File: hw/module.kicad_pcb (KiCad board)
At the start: 2 copper layers, 30 x 30 mm, 1 part

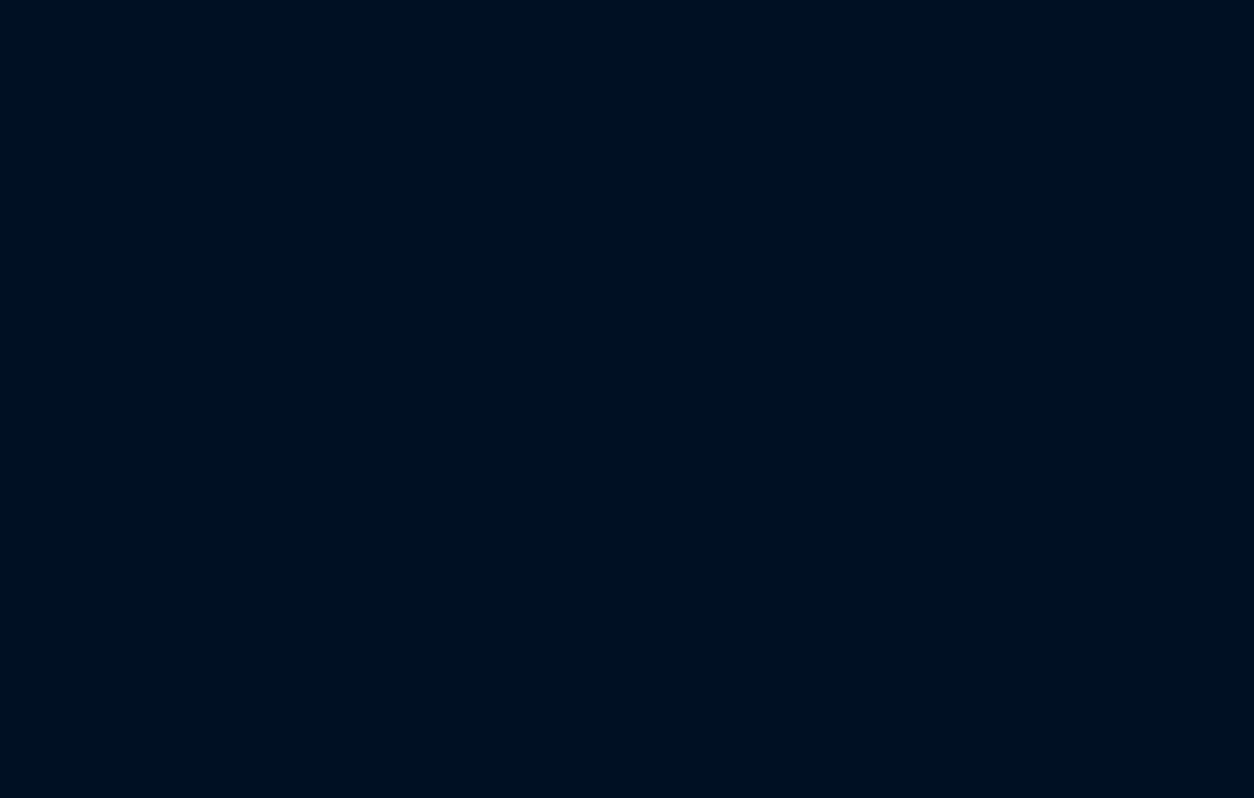
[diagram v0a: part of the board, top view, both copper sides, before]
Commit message: Footprint assignment
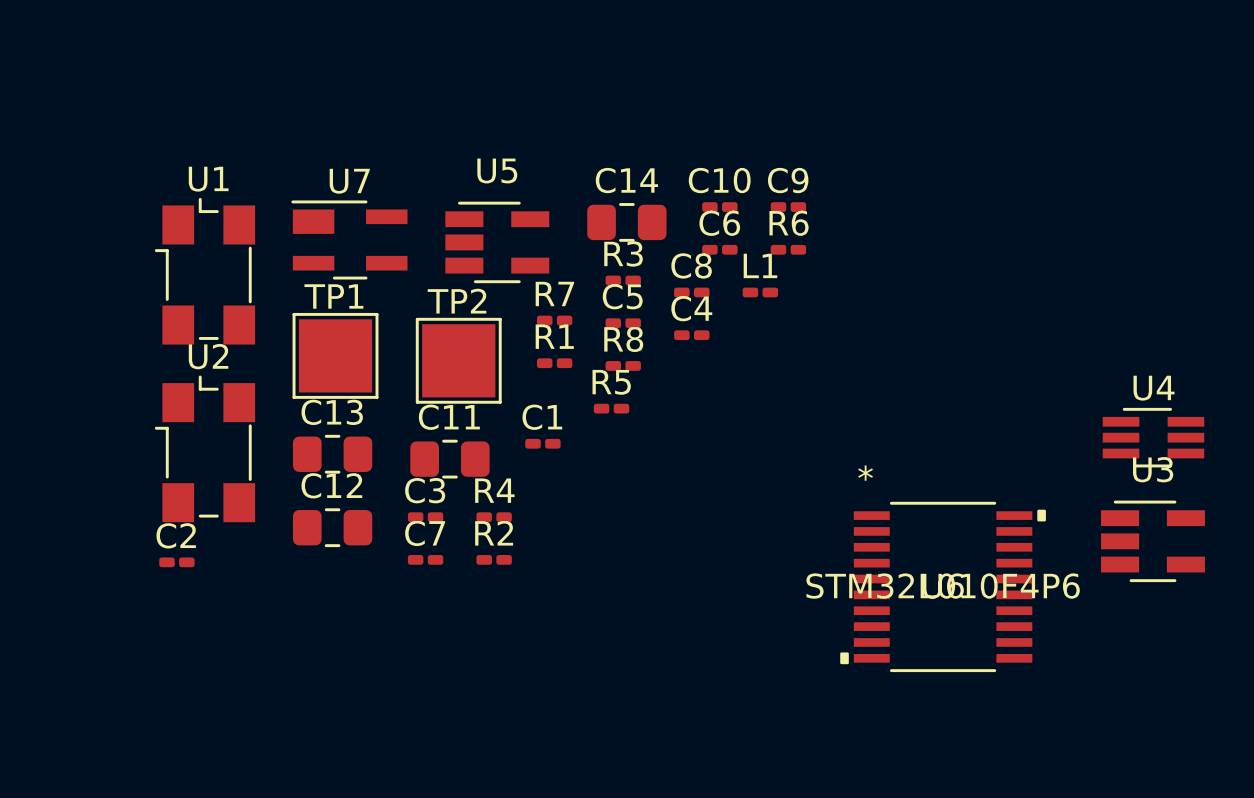
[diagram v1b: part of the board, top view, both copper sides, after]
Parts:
- added C1: 10n, Capacitor_SMD:C_0201_0603Metric_Pad0.64x0.40mm_HandSolder, F.Cu at (99.5, 62.5)
- added C10: 10n, Capacitor_SMD:C_0201_0603Metric_Pad0.64x0.40mm_HandSolder, F.Cu at (106.8, 52.8)
- added C11: 100n, Capacitor_SMD:C_0805_2012Metric_Pad1.18x1.45mm_HandSolder, F.Cu at (95.7, 63.1)
- added C12: 100n, Capacitor_SMD:C_0805_2012Metric_Pad1.18x1.45mm_HandSolder, F.Cu at (90.9, 65.9)
- added C13: 100n, Capacitor_SMD:C_0805_2012Metric_Pad1.18x1.45mm_HandSolder, F.Cu at (90.9, 62.9)
- added C14: 100n, Capacitor_SMD:C_0805_2012Metric_Pad1.18x1.45mm_HandSolder, F.Cu at (102.9, 53.4)
- added C2: 10n, Capacitor_SMD:C_0201_0603Metric_Pad0.64x0.40mm_HandSolder, F.Cu at (84.5, 67.4)
- added C3: 100n, Capacitor_SMD:C_0201_0603Metric_Pad0.64x0.40mm_HandSolder, F.Cu at (94.7, 65.5)
- added C4: 100n, Capacitor_SMD:C_0201_0603Metric_Pad0.64x0.40mm_HandSolder, F.Cu at (105.6, 58.0)
- added C5: 200p, Capacitor_SMD:C_0201_0603Metric_Pad0.64x0.40mm_HandSolder, F.Cu at (102.8, 57.6)
- added C6: 200p, Capacitor_SMD:C_0201_0603Metric_Pad0.64x0.40mm_HandSolder, F.Cu at (106.8, 54.5)
- added C7: 10n, Capacitor_SMD:C_0201_0603Metric_Pad0.64x0.40mm_HandSolder, F.Cu at (94.7, 67.3)
- added C8: 100n, Capacitor_SMD:C_0201_0603Metric_Pad0.64x0.40mm_HandSolder, F.Cu at (105.6, 56.3)
- added C9: 100n, Capacitor_SMD:C_0201_0603Metric_Pad0.64x0.40mm_HandSolder, F.Cu at (109.6, 52.8)
- added L1: L, Inductor_SMD:L_0201_0603Metric_Pad0.64x0.40mm_HandSolder, F.Cu at (108.4, 56.3)
- added R1: 10k, Resistor_SMD:R_0201_0603Metric_Pad0.64x0.40mm_HandSolder, F.Cu at (100.0, 59.2)
- added R2: 10k, Resistor_SMD:R_0201_0603Metric_Pad0.64x0.40mm_HandSolder, F.Cu at (97.5, 67.3)
- added R3: 800k, Resistor_SMD:R_0201_0603Metric_Pad0.64x0.40mm_HandSolder, F.Cu at (102.8, 55.8)
- added R4: 800k, Resistor_SMD:R_0201_0603Metric_Pad0.64x0.40mm_HandSolder, F.Cu at (97.5, 65.5)
- added R5: R, Resistor_SMD:R_0201_0603Metric_Pad0.64x0.40mm_HandSolder, F.Cu at (102.3, 61.1)
- added R6: 500k, Resistor_SMD:R_0201_0603Metric_Pad0.64x0.40mm_HandSolder, F.Cu at (109.6, 54.5)
- added R7: 500k, Resistor_SMD:R_0201_0603Metric_Pad0.64x0.40mm_HandSolder, F.Cu at (100.0, 57.5)
- added R8: 10k, Resistor_SMD:R_0201_0603Metric_Pad0.64x0.40mm_HandSolder, F.Cu at (102.8, 59.3)
- added TP1: SWDIO, TestPoint:TestPoint_Pad_3.0x3.0mm, F.Cu at (91.0, 58.9)
- added TP2: SWCLK, TestPoint:TestPoint_Pad_3.0x3.0mm, F.Cu at (96.0, 59.1)
- added U1: CFPS-39, Oscillator:Oscillator_SMD_Fox_FT5H_5.0x3.2mm, F.Cu at (85.8, 55.6)
- added U2: CFPS-39, Oscillator:Oscillator_SMD_Fox_FT5H_5.0x3.2mm, F.Cu at (85.8, 62.9)
- added U3: 74LVC1G125, Package_TO_SOT_SMD:SOT-23-5_HandSoldering, F.Cu at (124.5, 66.5)
- added U4: mux, Package_TO_SOT_SMD:SOT-363_SC-70-6_Handsoldering, F.Cu at (124.5, 62.2)
- added U5: MAX919, Package_TO_SOT_SMD:SOT-23-5_HandSoldering, F.Cu at (97.6, 54.2)
- added U6: STM32L010F4P6, farnell:STM32L010F4P6, F.Cu at (115.9, 68.4)
- added U7: BAS70-7-F, Package_TO_SOT_SMD:SOT-143_Handsoldering, F.Cu at (91.6, 54.1)

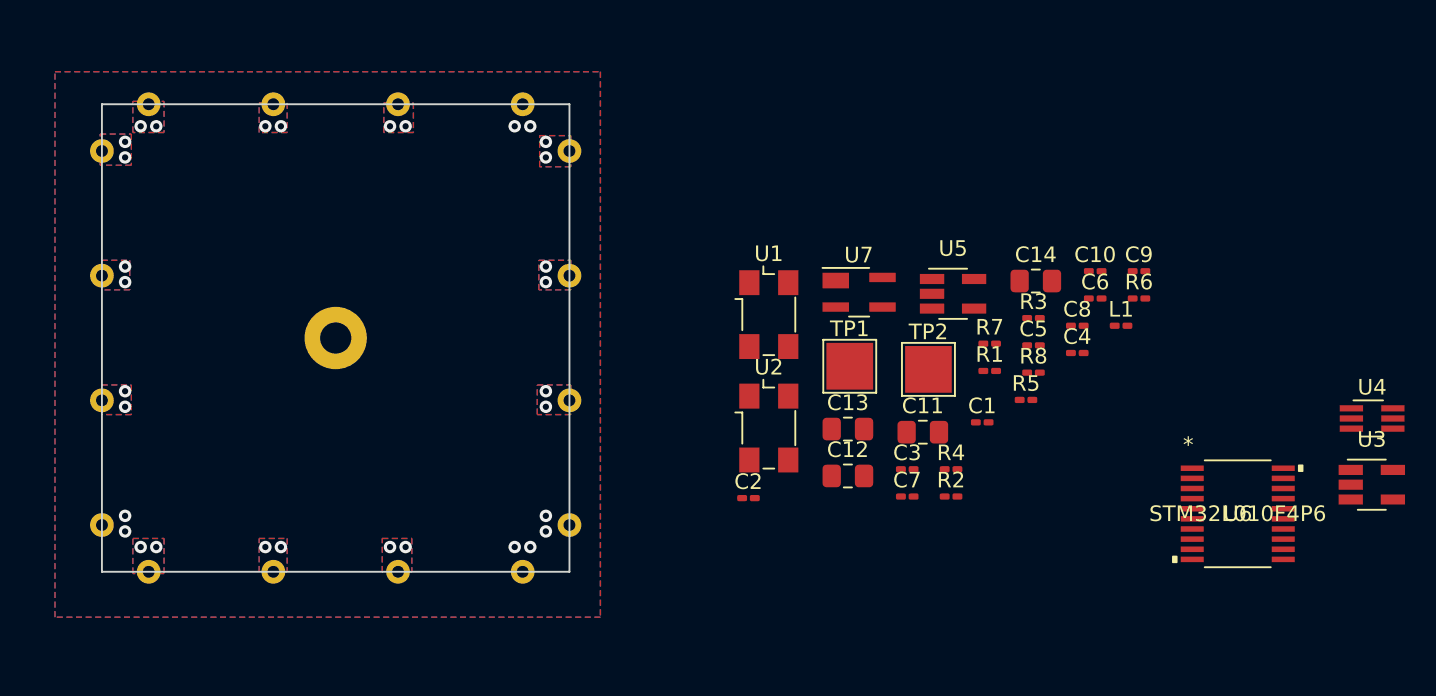
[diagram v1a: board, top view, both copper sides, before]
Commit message: PCB arrange
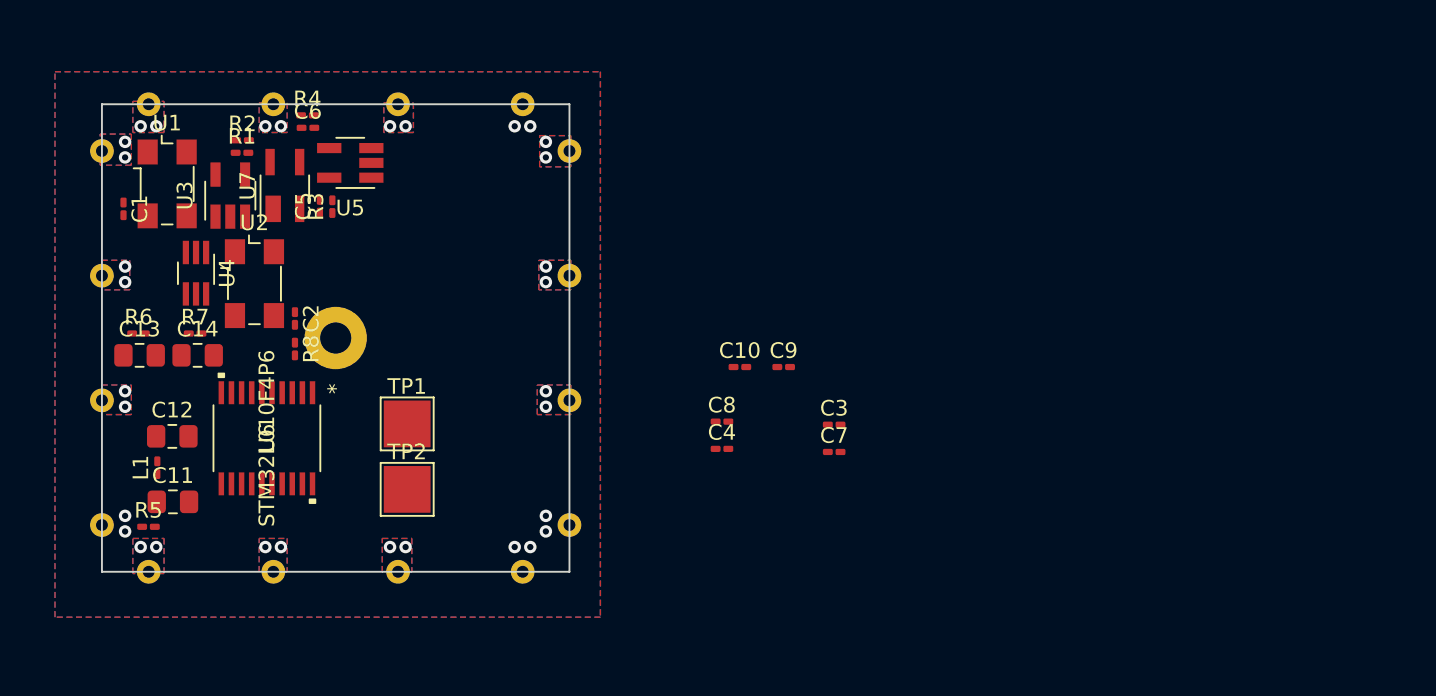
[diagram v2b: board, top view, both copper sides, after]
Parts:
- moved U4 76.0 mm to (49.0, 52.9), turned to -90 degrees
- moved U3 75.6 mm to (51.2, 48.0), turned to 90 degrees
- moved R6 64.2 mm to (45.4, 56.8)
- moved L1 62.5 mm to (46.6, 65.4), turned to 90 degrees
- moved U6 62.5 mm to (53.6, 63.5), turned to -90 degrees
- moved R5 56.9 mm to (46.0, 69.2)
- moved C1 56.8 mm to (44.4, 48.8), turned to -90 degrees
- moved C14 54.0 mm to (49.2, 58.2)
- moved C6 51.7 mm to (56.2, 43.6)
- moved R7 51.0 mm to (49.0, 56.8)
- moved R2 50.9 mm to (52.0, 44.4)
- moved R1 50.0 mm to (52.0, 45.2)
- moved C11 48.3 mm to (47.6, 67.6)
- moved R8 47.4 mm to (55.4, 57.8), turned to -90 degrees
- moved R4 47.1 mm to (56.2, 42.8)
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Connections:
- U7 pad 1: Net-(C6-Pad1) -> Net-(R1-Pad2)
- U7 pad 2: Net-(R1-Pad2) -> Net-(C6-Pad1)
- U7 pad 3: Net-(C5-Pad2) -> Net-(R2-Pad2)
- U7 pad 4: Net-(R2-Pad2) -> Net-(C5-Pad2)

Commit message: PCB wiring
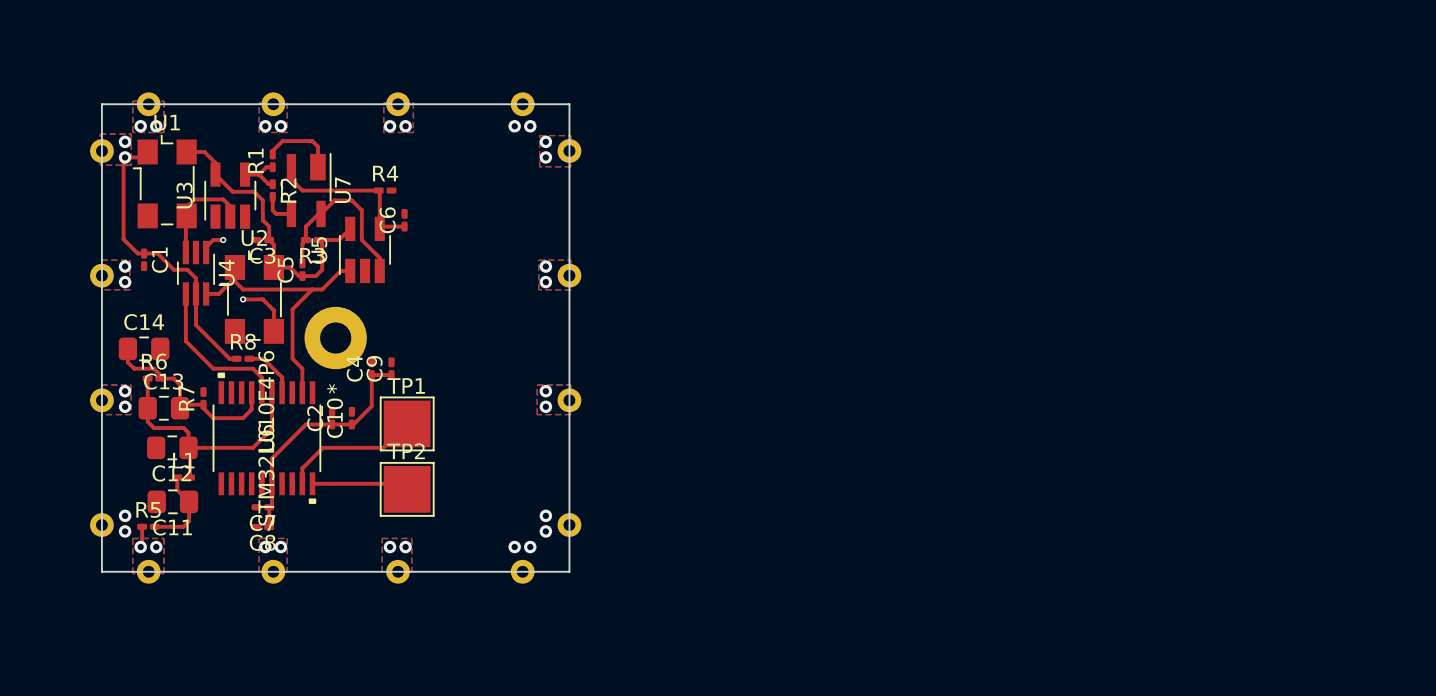
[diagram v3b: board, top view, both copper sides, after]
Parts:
- moved C3 38.5 mm to (53.3, 50.8), turned to 180 degrees
- moved C7 36.8 mm to (53.3, 67.9), turned to 180 degrees
- moved C8 30.2 mm to (53.3, 69.2), turned to 180 degrees
- moved C9 25.2 mm to (61.6, 59.1), turned to 90 degrees
- moved C10 25.1 mm to (59.1, 62.2), turned to 90 degrees
- moved C4 23.1 mm to (60.3, 59.1), turned to 90 degrees
- moved C6 8.58 mm to (62.4, 49.5), turned to 90 degrees
- moved R4 6.94 mm to (61.2, 47.6)
- moved C2 6.83 mm to (57.8, 62.2), turned to 90 degrees
- moved U5 5.66 mm to (59.9, 51.4), turned to 90 degrees
- moved C5 4.22 mm to (55.9, 52.7)
- moved R7 4.19 mm to (49.5, 61.0), turned to 90 degrees
- moved R2 3.76 mm to (54.0, 47.6), turned to -90 degrees
- moved C13 3.74 mm to (47.0, 61.6)
- moved C1 3.53 mm to (45.7, 52.1)
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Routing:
- net +3.3V: track 0.00 -> 55.4 mm
- net /OSC_STAT: track 0.00 -> 19.5 mm
- net +3.3VA: track 0.00 -> 16.8 mm
- net /half_vref: track 0.00 -> 12.9 mm
- net Net-(C5-Pad2): track 0.00 -> 11.5 mm
- net Net-(C6-Pad1): track 0.00 -> 10.8 mm
- net /OSC: track 0.00 -> 9.85 mm
- net Net-(TP1-Pad1): track 0.00 -> 8.89 mm
- net Net-(U1-Pad3): track 0.00 -> 6.77 mm
- net Net-(TP2-Pad1): track 0.00 -> 6.22 mm
- net Net-(C11-Pad1): track 0.00 -> 5.46 mm
- net Net-(U2-Pad3): track 0.00 -> 5.24 mm
- net Net-(R1-Pad2): track 0.00 -> 4.85 mm
- net Net-(R8-Pad2): track 0.00 -> 3.58 mm
- net Net-(R1-Pad1): track 0.00 -> 3.29 mm
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- removed copper zone on B.Cu, net GND
- removed copper zone on F.Cu, net GND

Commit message: Pcb++
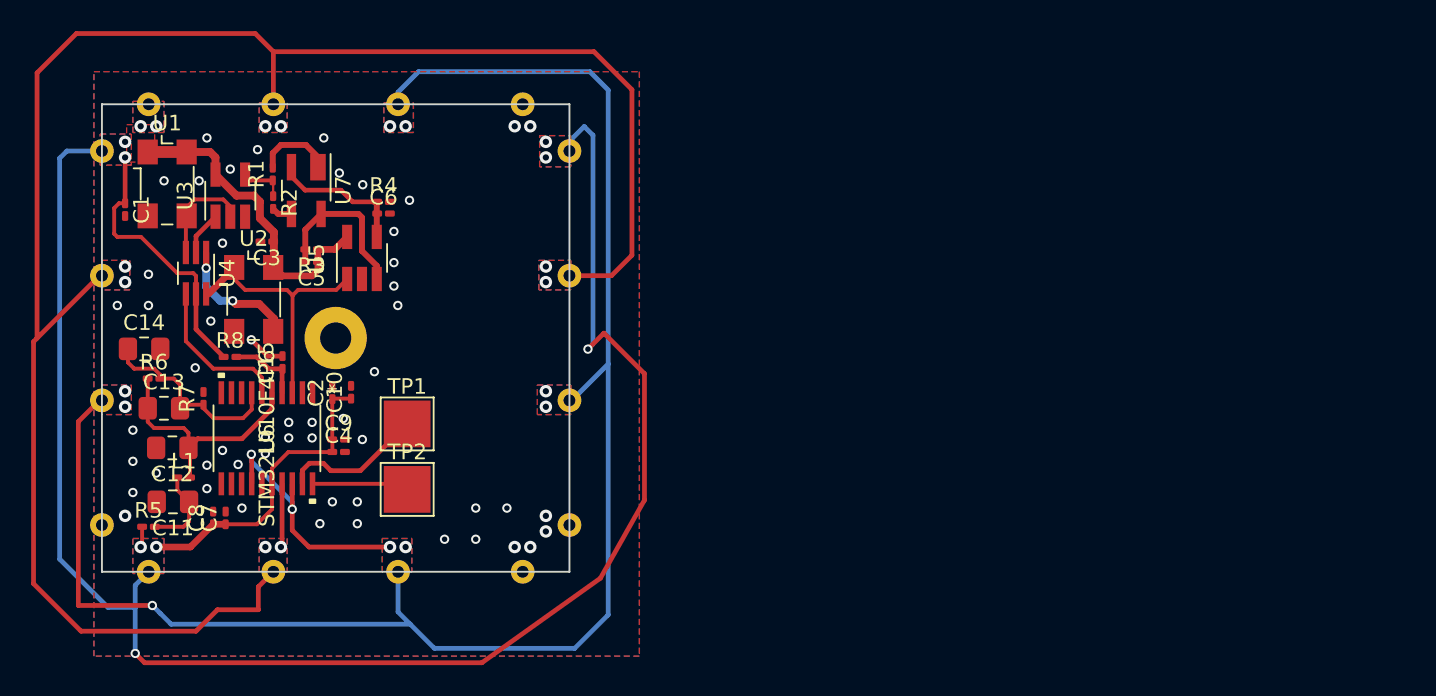
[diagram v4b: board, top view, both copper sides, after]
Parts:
- added C15: 1n, Capacitor_SMD:C_0201_0603Metric_Pad0.64x0.40mm_HandSolder, F.Cu at (54.6, 58.7)
- U4: value mux -> 74 LVC 1G3157GW,125
- moved C4 5.75 mm to (58.2, 64.4), turned to 0 degrees
- moved C9 5.67 mm to (58.2, 63.6), turned to 0 degrees
- moved C1 3.44 mm to (44.5, 48.9)
- moved C8 3.24 mm to (50.1, 68.6), turned to 90 degrees
- moved C7 2.49 mm to (51.0, 68.6), turned to 90 degrees
- moved C10 1.66 mm to (59.0, 60.6)
- moved C2 1.63 mm to (57.8, 60.6)
- moved C6 1.42 mm to (61.1, 49.1), turned to 0 degrees
- moved R1 0.85 mm to (54.0, 46.6)
- moved R8 0.85 mm to (51.2, 58.3)
- moved C5 0.77 mm to (56.5, 52.2), turned to 180 degrees
- moved R2 0.77 mm to (54.0, 48.4)
- moved R4 0.73 mm to (61.1, 48.4)
- moved R3 0.60 mm to (56.5, 51.4)
- moved U5 0.55 mm to (59.7, 52.0)
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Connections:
- U6 pad 14: unconnected-(U6-Pad14) -> /RX
- U6 pad 17: /RX -> /TX
- U6 pad 18: /TX -> /RX
- U6 pad 2: /OSC_STAT -> unconnected-(U6-Pad2)
- U6 pad 3: unconnected-(U6-Pad3) -> /OSC_STAT
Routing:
- net /RX: track 0.00 -> 121.6 mm, vias 8 -> 11
- net /TX: track 0.00 -> 120.6 mm
- net +3.3V: track 55.4 -> 167.4 mm, vias 8 -> 10
- net GND: track 0.00 -> 5.25 mm, vias 8 -> 53
- net Net-(U2-Pad3): track 5.24 -> 8.21 mm, vias 0 -> 2
- net /OSC_STAT: track 19.5 -> 17.5 mm
- net Net-(C6-Pad1): track 10.8 -> 9.36 mm
- net Net-(R8-Pad2): track 3.58 -> 4.82 mm
- net Net-(C5-Pad2): track 11.5 -> 10.6 mm
- net Net-(R2-Pad2): track 2.16 -> 1.31 mm
- net +3.3VA: track 16.8 -> 16.0 mm
- net (no net): vias 2 -> 0
- added copper zone on B.Cu, net GND
- added copper zone on F.Cu, net GND
